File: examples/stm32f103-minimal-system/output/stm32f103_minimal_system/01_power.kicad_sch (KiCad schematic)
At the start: 8 parts, among them J1 USB-C16PIN, U2 AMS1117-3.3

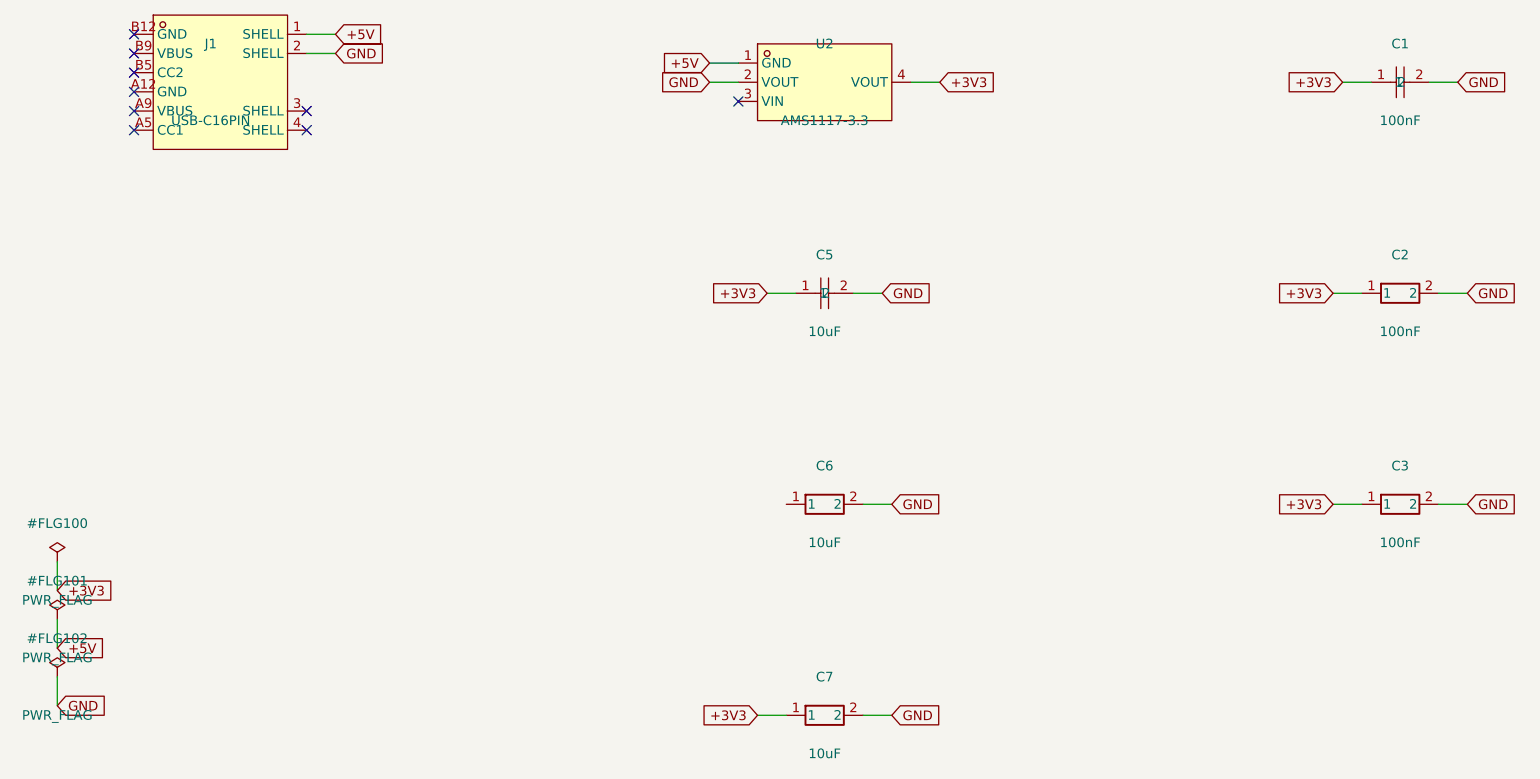
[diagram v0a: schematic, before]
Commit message: docs: refresh verified examples / 文档：刷新已验证示例
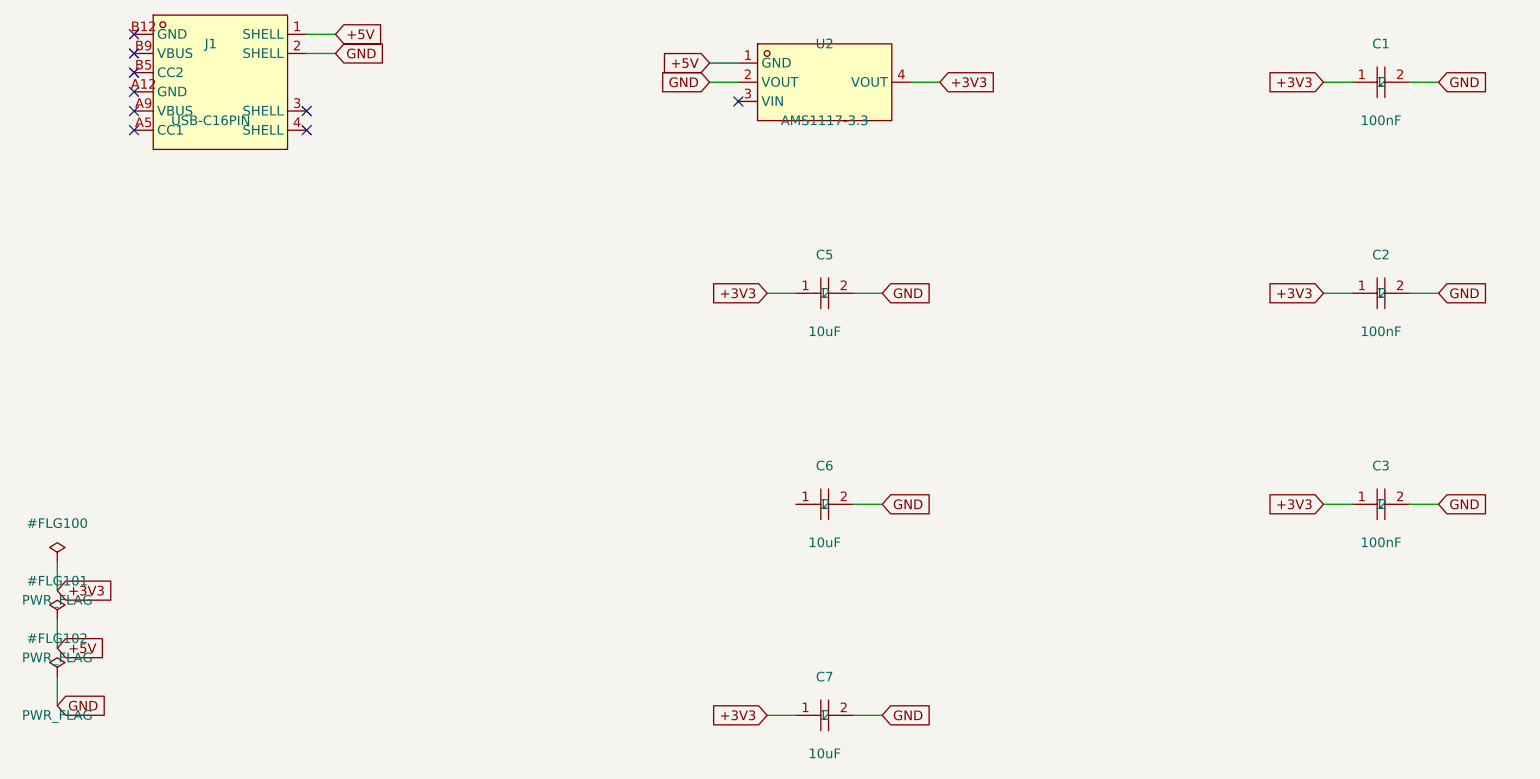
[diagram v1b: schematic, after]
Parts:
- removed C2, C3: 100nF, symbol JLC-MCP:C1590
- removed C6, C7: 10uF, symbol JLC-MCP:C1713
- added C2, C3: 100nF, JLC-MCP:C0603, symbol JLC-MCP:CL10B104KA8NNNC
- added C6, C7: 10uF, JLC-MCP:C0805, symbol JLC-MCP:CL21A106KOQNNNE
- C1: footprint (none) -> JLC-MCP:C0603
- C5: footprint (none) -> JLC-MCP:C0805
- J1: footprint (none) -> JLC-MCP:USB-C-SMD_USB-TYPE-C-006
- U2: footprint (none) -> JLC-MCP:SOT-223-3_L6.5-W3.4-P2.30-LS7.0-BR
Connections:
- net +3V3: now also C2.1, C3.1, C7.1
- net GND: now also C2.2, C3.2, C6.2, C7.2
